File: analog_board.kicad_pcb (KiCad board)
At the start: 2 copper layers, 80 x 80 mm, 48 parts, among them J301 SAMTEC-TSW-105-07-X-D, J302 SAMTEC-TSW-105-07-X-D, J304 SAMTEC-TSW-105-07-X-D, J305 SAMTEC-TSW-105-07-X-D, U1 LM324, U3 AD620, U4 AD620

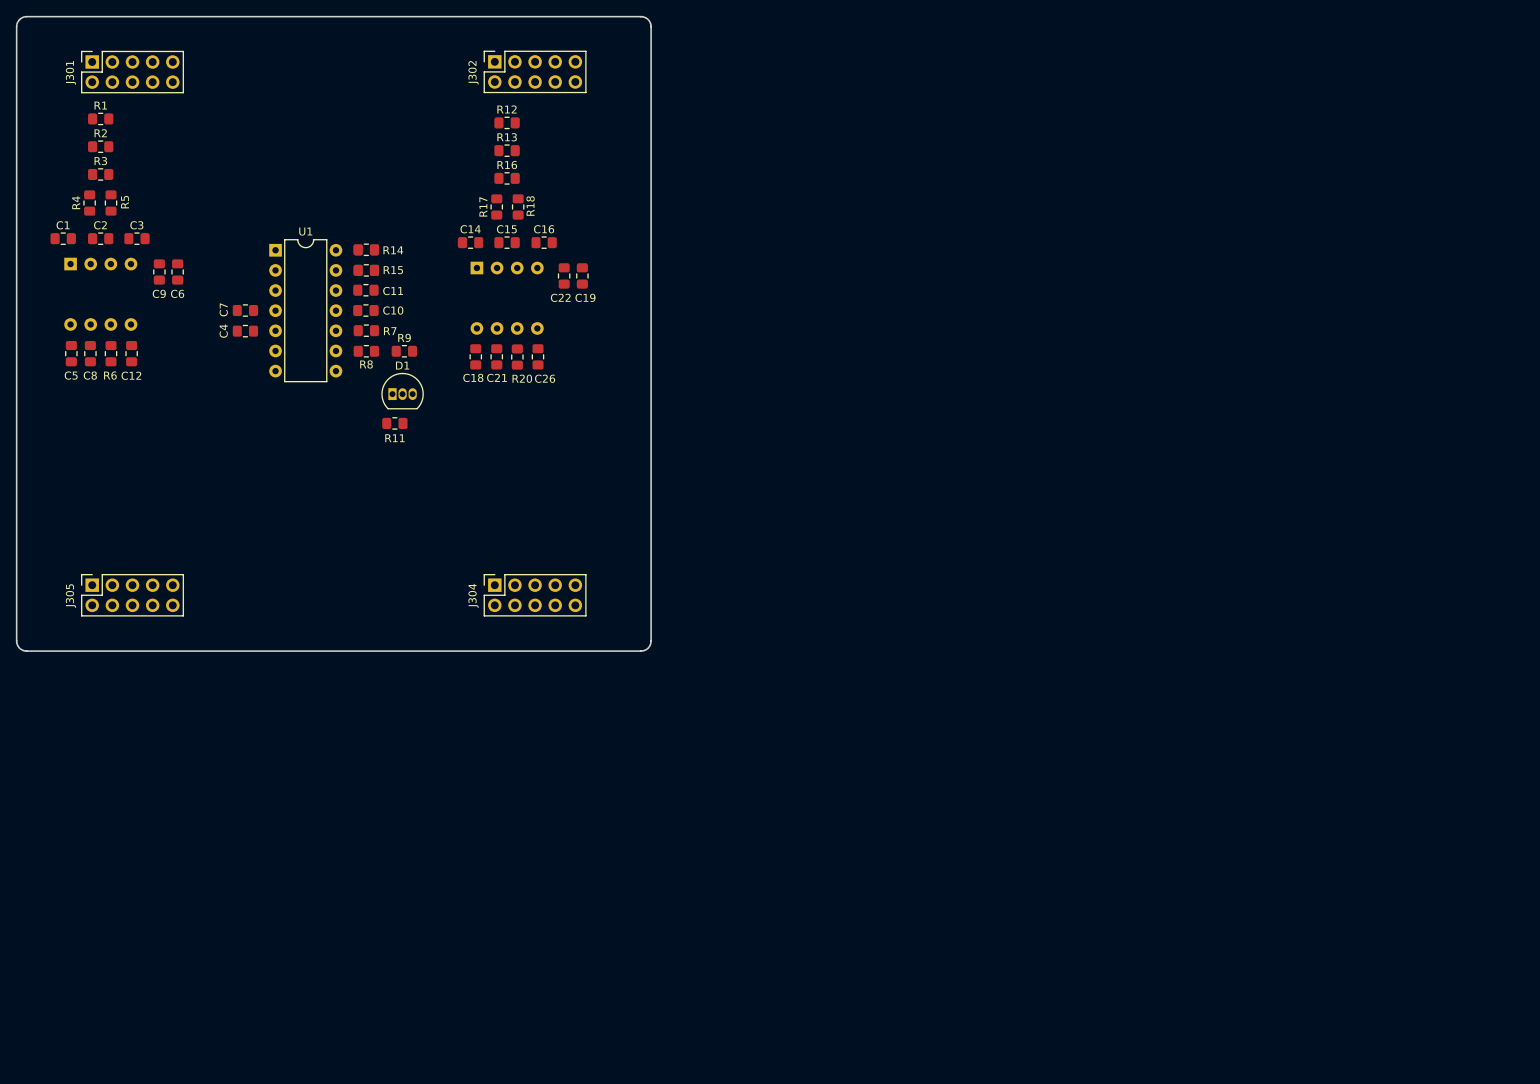
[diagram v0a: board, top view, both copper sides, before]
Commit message: Most wiring is done, no ground yet
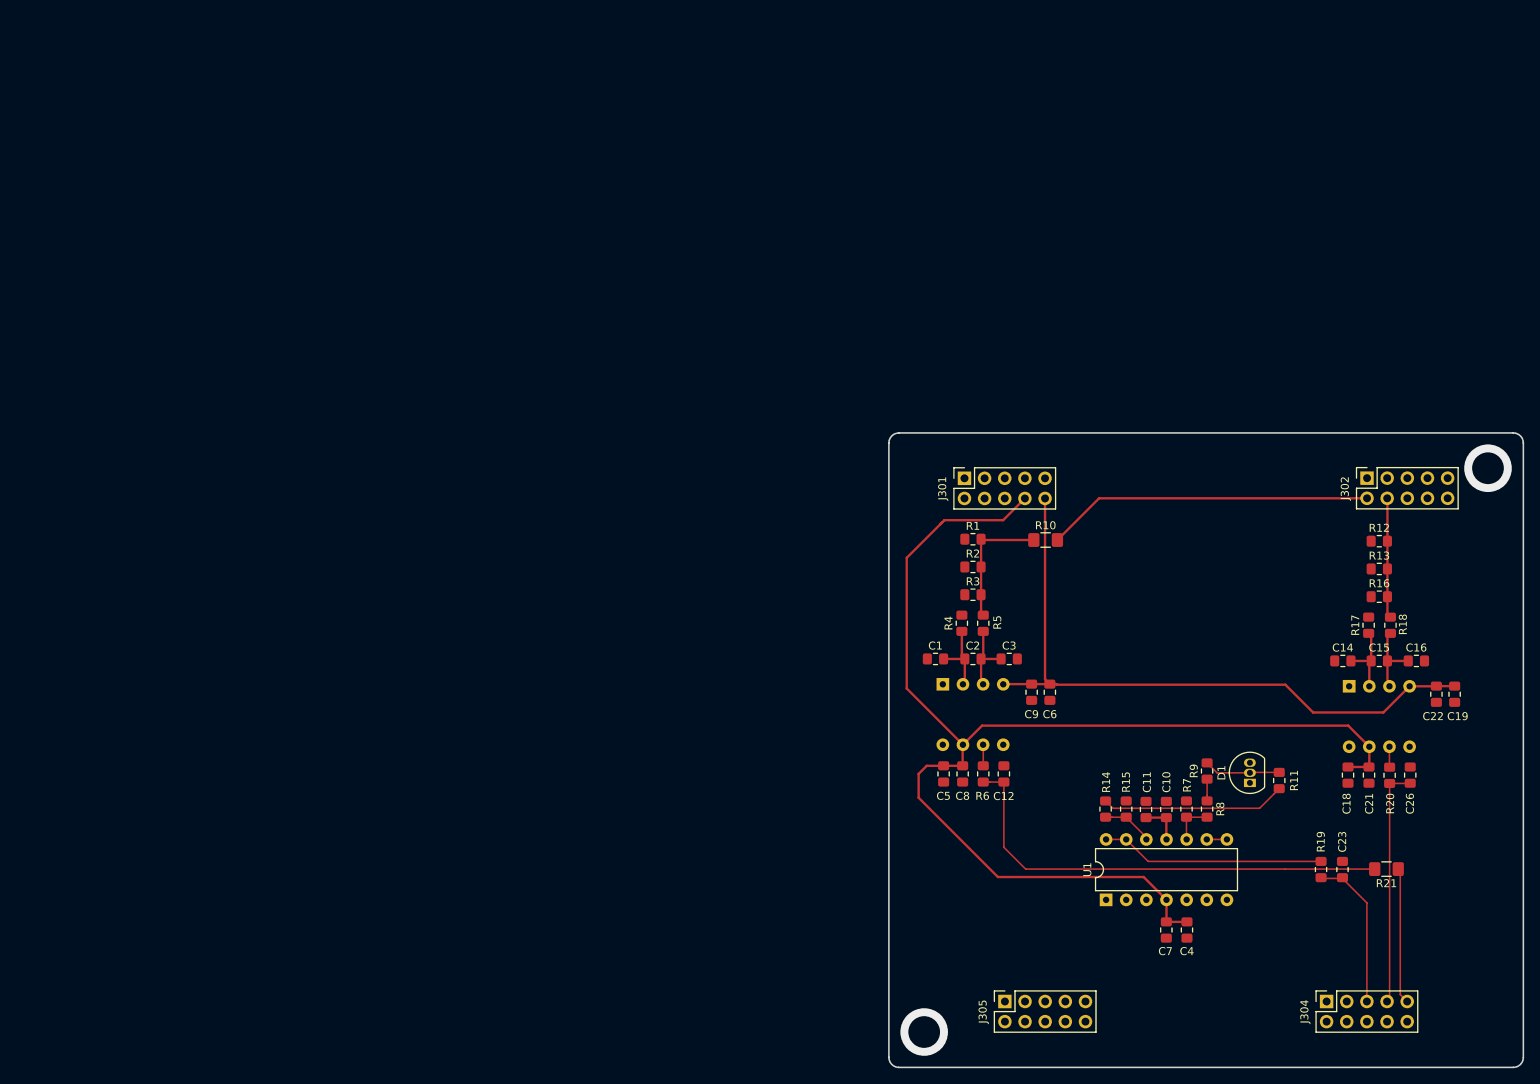
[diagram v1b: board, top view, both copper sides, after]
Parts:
- added R10: 0R, Resistor_SMD:R_1206_3216Metric_Pad1.42x1.75mm_HandSolder, F.Cu at (129.8, 66.0)
- added R21: 0R, Resistor_SMD:R_1206_3216Metric_Pad1.42x1.75mm_HandSolder, F.Cu at (172.8, 107.5)
- C23, R19: moved to F.Cu
- moved C23 144.4 mm to (167.2, 107.6), turned to 90 degrees
- moved R19 143.5 mm to (164.5, 107.6), turned to 90 degrees
- moved C4 140.7 mm to (147.6, 115.2), turned to 270 degrees
- moved C7 140.0 mm to (145.0, 115.2), turned to 270 degrees
- moved U1 133.0 mm to (137.4, 111.4), turned to 90 degrees
- moved J305 126.5 mm to (124.6, 124.2)
- moved C6 122.1 mm to (130.3, 85.2)
- moved C1 122.1 mm to (115.9, 81.0)
- moved C12 122.1 mm to (124.5, 95.5)
- moved C2 122.1 mm to (120.6, 81.0)
- moved C3 122.1 mm to (125.2, 81.0)
- moved C5 122.1 mm to (116.9, 95.5)
- moved C8 122.1 mm to (119.3, 95.5)
- moved C9 122.1 mm to (128.0, 85.2)
- moved R1 122.1 mm to (120.6, 65.9)
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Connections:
- C12 pad 1: /Current_ch1_out -> Net-(C12-Pad1)
- R1 pad 2: /Current_sensor_1 -> Net-(R1-Pad2)
- R2 pad 2: /Current_sensor_1 -> Net-(R1-Pad2)
- R3 pad 2: /Current_sensor_1 -> Net-(R1-Pad2)
- R5 pad 2: /Current_sensor_1 -> Net-(R1-Pad2)
- R6 pad 1: /Current_ch1_out -> Net-(C12-Pad1)
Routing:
- net +15V: track 0.00 -> 157.0 mm
- net -15V: track 0.00 -> 88.8 mm
- net Net-(C12-Pad1): track 0.00 -> 59.0 mm
- net /Current_sensor_1: track 0.00 -> 41.2 mm
- net /Current_ch2_out: track 0.00 -> 30.2 mm
- net Net-(R19-Pad2): track 0.00 -> 28.3 mm
- net /3V3_REF: track 0.00 -> 23.3 mm
- net /Torque_pedal_ADC: track 0.00 -> 19.5 mm
- net /Current_ch1_out: track 0.00 -> 17.1 mm
- net Net-(R1-Pad2): track 0.00 -> 16.4 mm
- net /Current_sensor_2: track 0.00 -> 15.2 mm
- net Net-(C15-Pad2): track 0.00 -> 10.1 mm
- net Net-(C14-Pad2): track 0.00 -> 9.84 mm
- net Net-(D1-Pad2): track 0.00 -> 9.64 mm
- net Net-(C1-Pad2): track 0.00 -> 9.60 mm
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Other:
- net class Current_sensor added: clearance 0.2, trace_width 0.3, via_dia 0.8, via_drill 0.4
- net class Default: clearance 0.15 -> 0.2; trace_width 0.15 -> 0.2
- net class Power: clearance 0.15 -> 0.2; trace_width 0.2 -> 0.3
- rule trace_clearance: 0.15 -> 0.2
